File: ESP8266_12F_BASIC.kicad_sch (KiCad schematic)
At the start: 39 parts, among them J1 Conn_01x02_Male, J2 Conn_01x04_Male, J3 Conn_01x05_Female, Q1 BC547, U1 ESP-12F, U2 AP1117-33

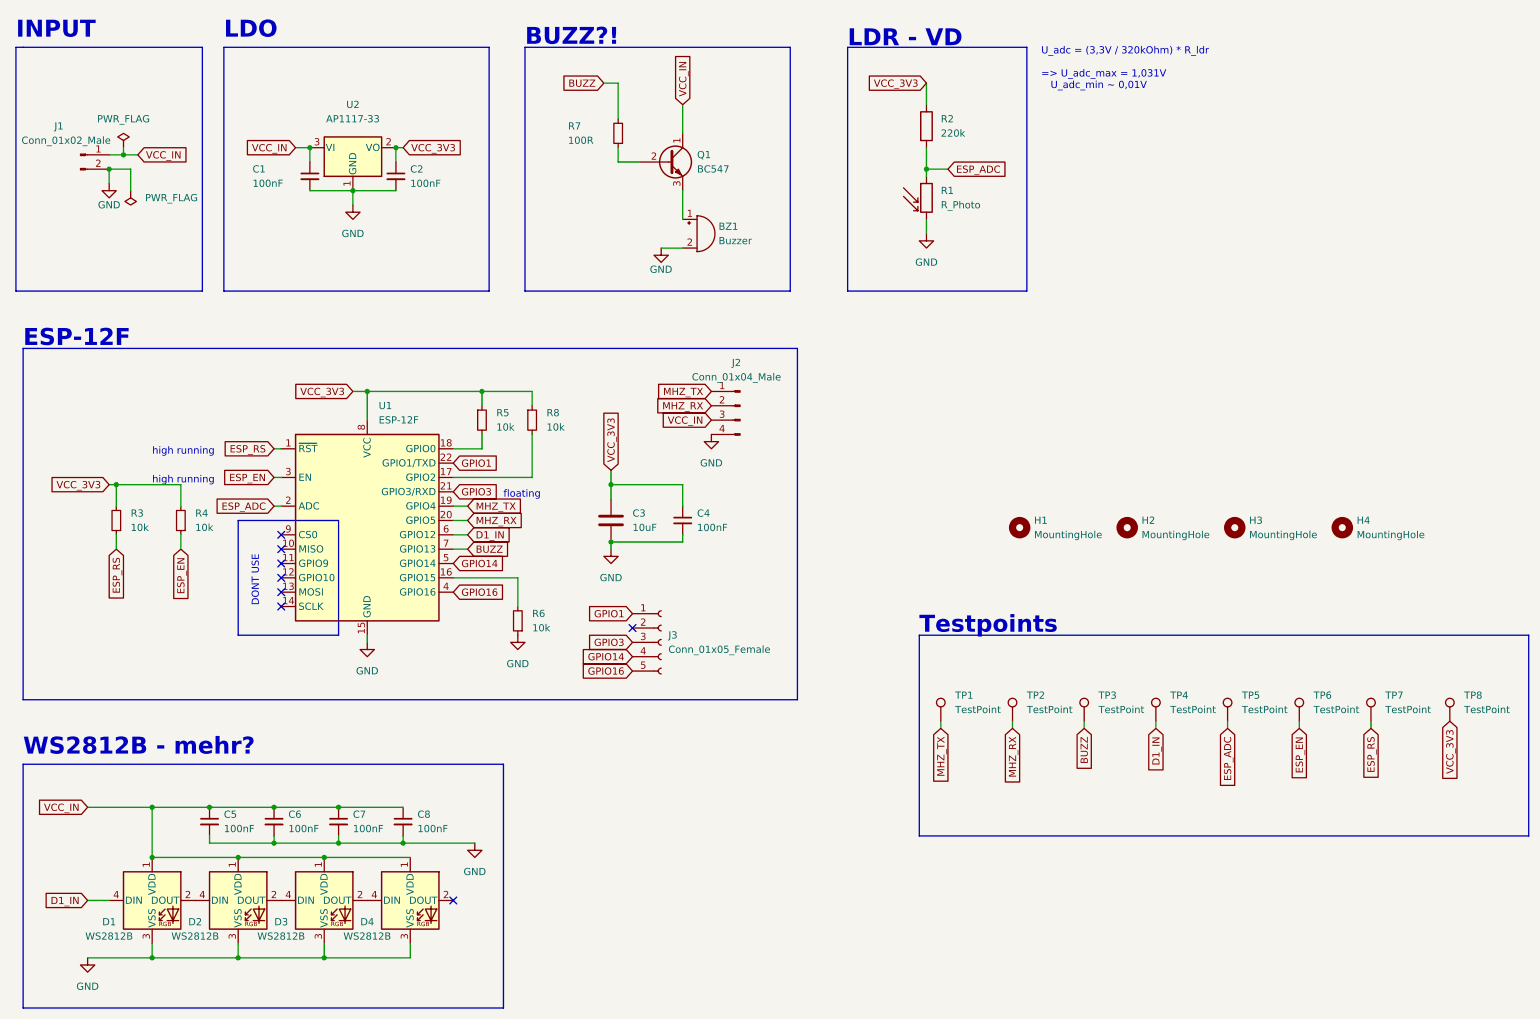
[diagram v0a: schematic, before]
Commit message: old state no hotfix
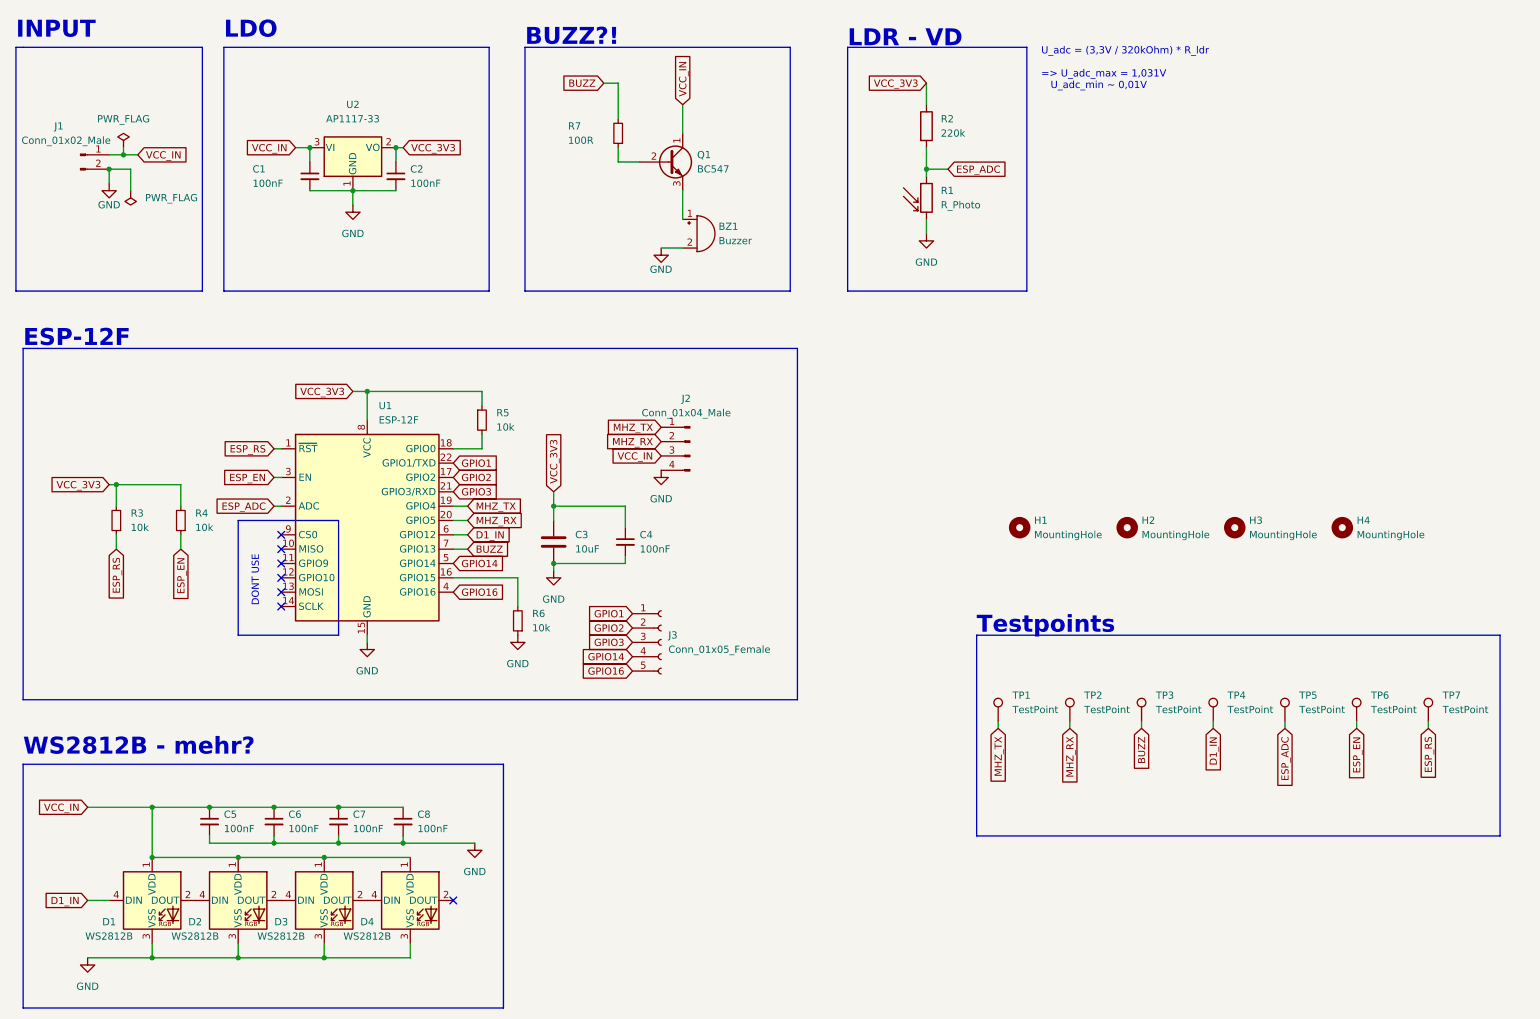
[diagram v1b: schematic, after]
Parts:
- removed R8: 10k, Resistor_SMD:R_0805_2012Metric_Pad1.20x1.40mm_HandSolder, symbol Device:R_Small
- removed TP8: TestPoint, TestPoint:TestPoint_THTPad_D3.0mm_Drill1.5mm, symbol Connector:TestPoint
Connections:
- net GPIO2: now reaches J3.2 (Pin_2)
- net GPIO2: now also U1.17 (GPIO2)
- no-connect marks 8 -> 7
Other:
- note removed: "floating"
- note removed: "high running"
- moved on the sheet: C3, C4, J2, TP1, TP2, TP3, TP4, TP5, TP6, TP7

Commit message: reset
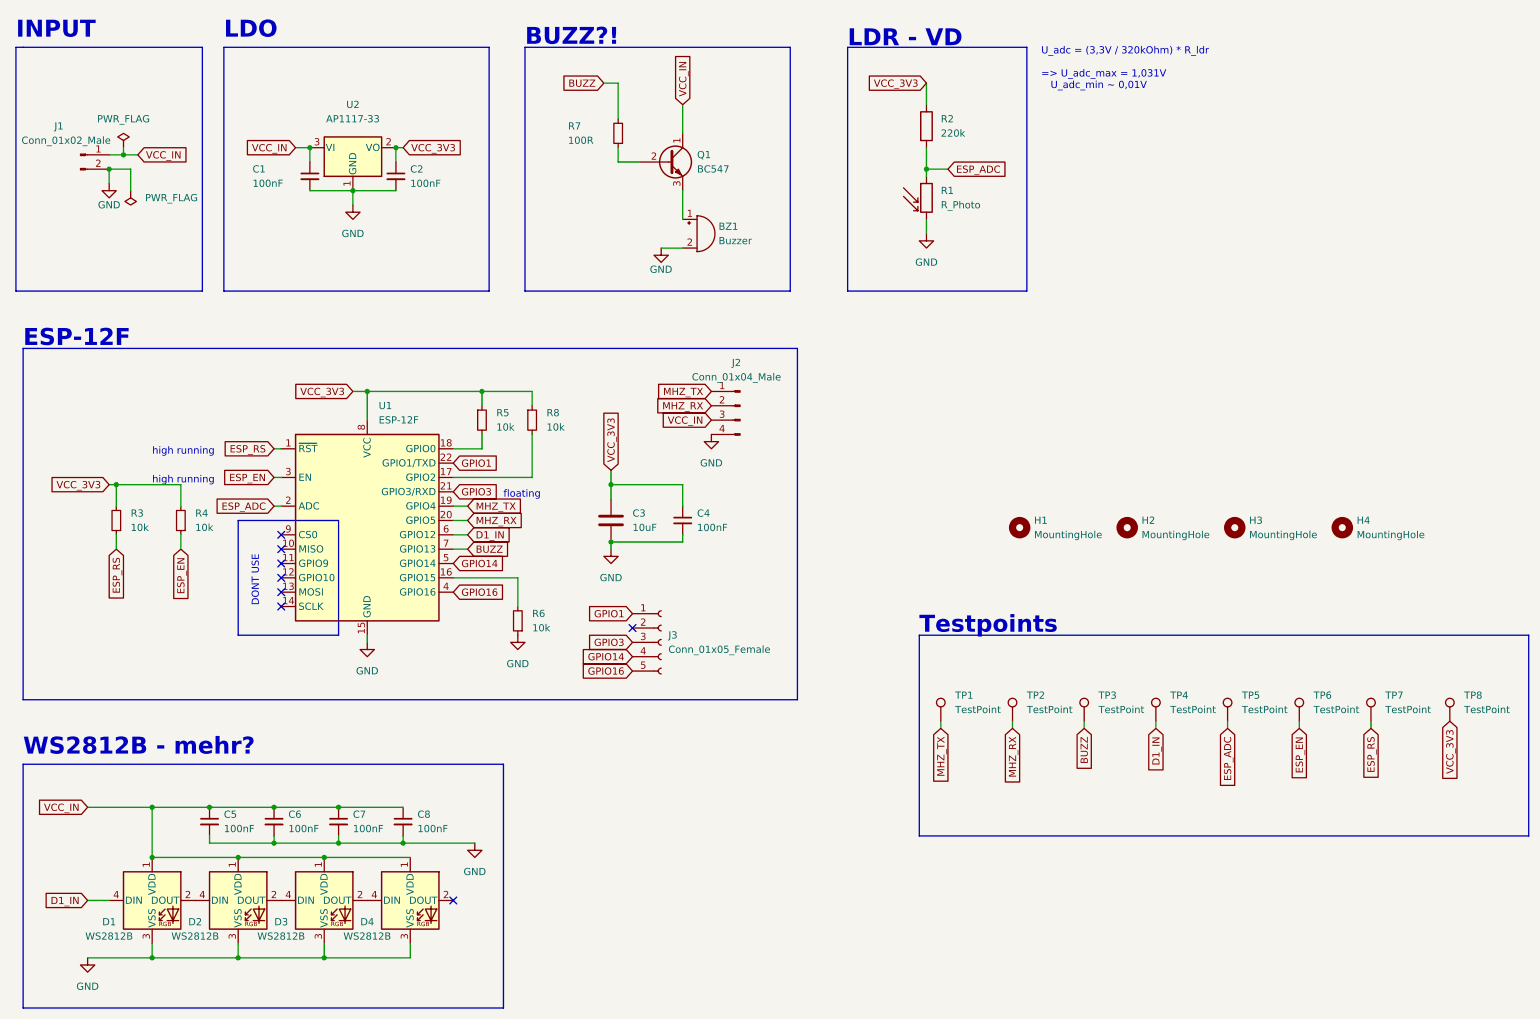
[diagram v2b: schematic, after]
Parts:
- added R8: 10k, Resistor_SMD:R_0805_2012Metric_Pad1.20x1.40mm_HandSolder, symbol Device:R_Small
- added TP8: TestPoint, TestPoint:TestPoint_THTPad_D3.0mm_Drill1.5mm, symbol Connector:TestPoint
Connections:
- net VCC_3V3: now also R8.1, TP8.1
- net GPIO2: no longer names the net of J3.2 (Pin_2)
- net GPIO2: no longer U1.17 (GPIO2)
- new net: R8.2, U1.17 (GPIO2)
- no-connect marks 7 -> 8
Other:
- note added: "floating"
- note added: "high running"
- moved on the sheet: C3, C4, J2, TP1, TP2, TP3, TP4, TP5, TP6, TP7
